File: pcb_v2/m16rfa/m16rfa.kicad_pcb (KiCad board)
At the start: 2 copper layers, 140.3 x 146.7 mm, 51 parts, among them J1 S16A, J10 bus_rf16_3, J2 S16A, J3 SWRDA, J5 S16A, J6 S16A, J7 S16A, J8 bus_rf16_1, J9 bus_rf16_2, U1 74LS125, U10 74LS244, U11 74LS244, U2 74LS193, U3 74LS138, U4 74LS08, U5 74LS04, U6 74LS08, U7 74LS244, U8 74LS244, U9 74LS244

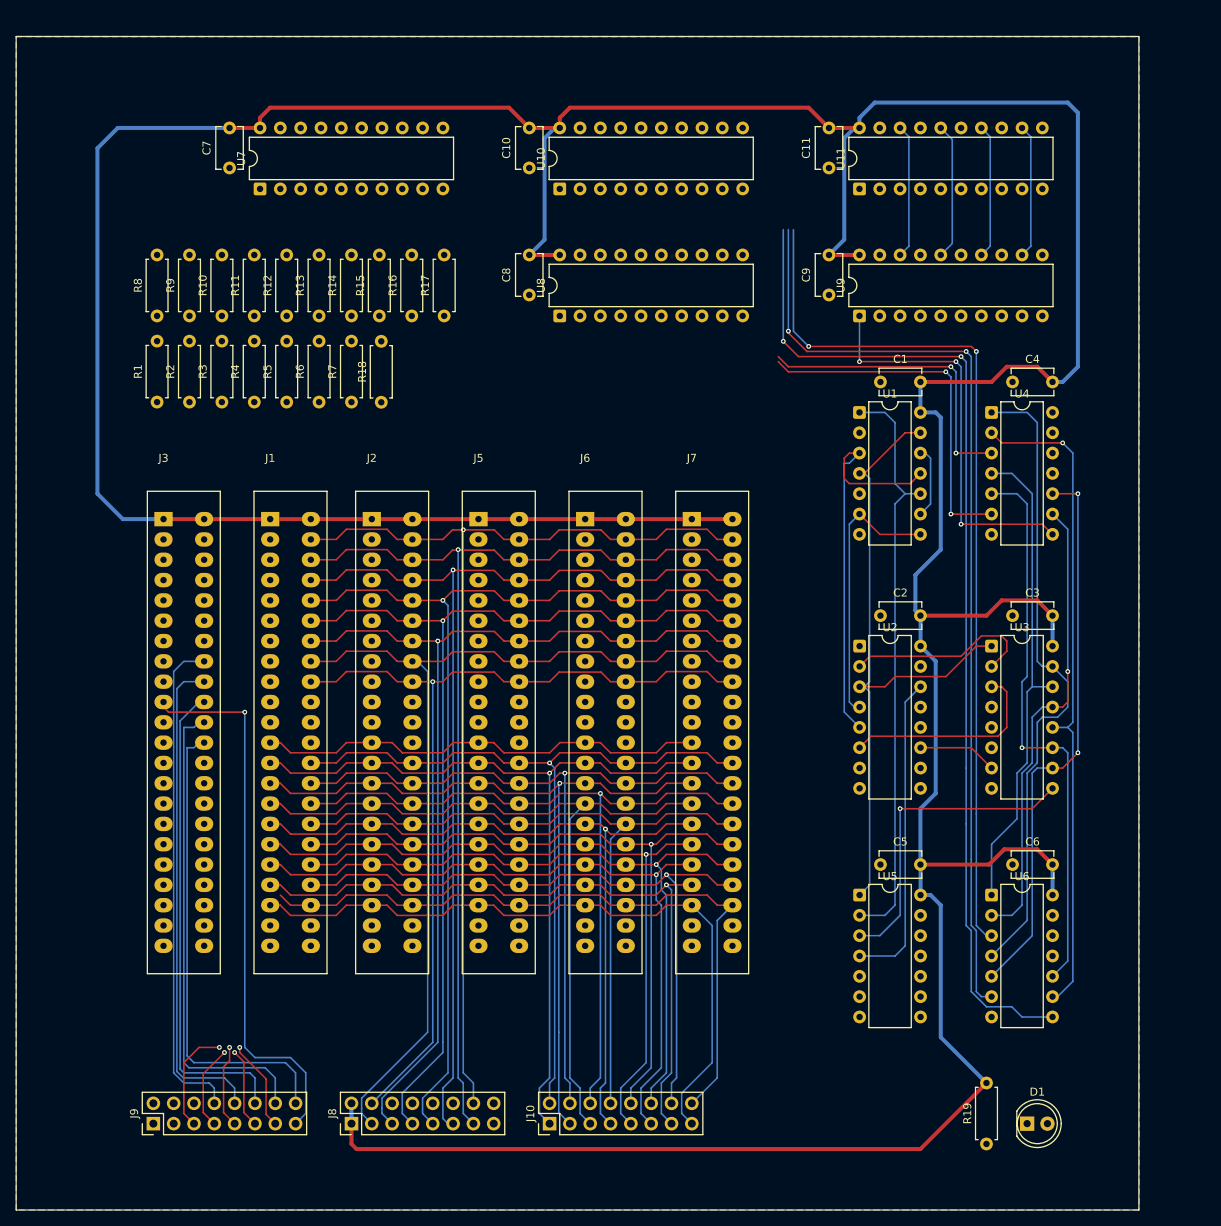
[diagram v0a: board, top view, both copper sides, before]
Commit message: recomeçando o roteamento
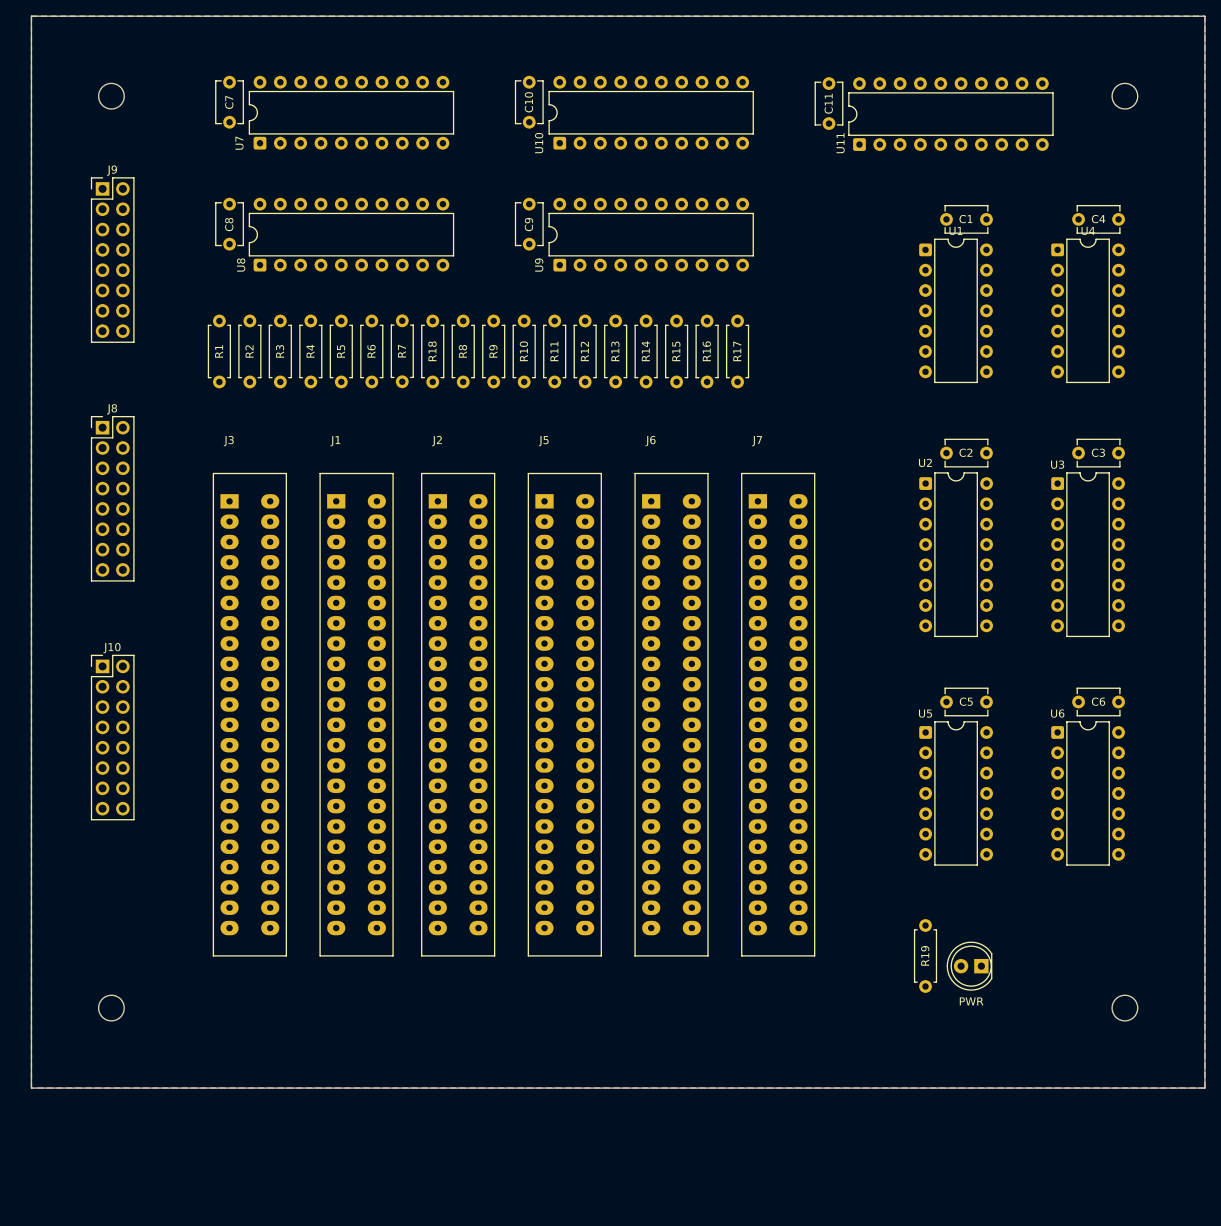
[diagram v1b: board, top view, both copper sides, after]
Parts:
- moved J9 117.0 mm to (36.8, 39.4), turned to 0 degrees
- moved J8 92.4 mm to (36.8, 69.2), turned to 0 degrees
- moved J10 79.9 mm to (36.8, 99.1), turned to 0 degrees
- moved R8 39.2 mm to (81.9, 63.5)
- moved R9 38.9 mm to (85.7, 63.5)
- moved R10 38.7 mm to (89.5, 63.5)
- moved R11 38.4 mm to (93.3, 63.5)
- moved R12 38.2 mm to (97.2, 63.5)
- moved R15 38.1 mm to (108.6, 63.5)
- moved C8 38.0 mm to (52.7, 46.3)
- moved C9 38.0 mm to (90.2, 46.3)
- moved U8 38.0 mm to (56.5, 48.9)
- moved U9 38.0 mm to (94.0, 48.9)
- moved R13 38.0 mm to (101.0, 63.5)
- moved R16 37.8 mm to (112.4, 63.5)
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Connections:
- J8 pad 11: data_{2} -> data_{5}
- J8 pad 13: data_{1} -> data_{6}
- J8 pad 14: data_{0} -> data_{7}
- J8 pad 3: data_{6} -> data_{1}
- J8 pad 4: data_{7} -> data_{0}
- J8 pad 5: data_{5} -> data_{2}
- J8 pad 7: data_{4} -> data_{3}
- J8 pad 9: data_{3} -> data_{4}
- U4 pad 12: unconnected-(U4-Pad12) -> +5V
- U4 pad 13: unconnected-(U4-Pad13) -> +5V
- U5 pad 11: unconnected-(U5-Pad11) -> +5V
- U5 pad 13: unconnected-(U5-Pad13) -> +5V
- U5 pad 5: unconnected-(U5-Pad5) -> +5V
- U5 pad 9: unconnected-(U5-Pad9) -> +5V
- U6 pad 12: unconnected-(U6-Pad12) -> +5V
- U6 pad 13: unconnected-(U6-Pad13) -> +5V
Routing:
- net +5V: track 582.5 -> 0.00 mm
- net data_{1}: track 130.0 -> 0.00 mm, vias 1 -> 0
- net data_{0}: track 129.7 -> 0.00 mm, vias 1 -> 0
- net data_{2}: track 128.7 -> 0.00 mm, vias 1 -> 0
- net lr_at_two: track 128.4 -> 0.00 mm, vias 2 -> 0
- net data_{3}: track 124.9 -> 0.00 mm, vias 1 -> 0
- net data_{4}: track 122.9 -> 0.00 mm, vias 1 -> 0
- net data_{5}: track 121.2 -> 0.00 mm, vias 1 -> 0
- net data_{6}: track 120.3 -> 0.00 mm
- net lr_at_one: track 118.8 -> 0.00 mm, vias 2 -> 0
- net data_{7}: track 113.3 -> 0.00 mm, vias 1 -> 0
- net lr_at_zero: track 110.8 -> 0.00 mm, vias 2 -> 0
- net addr_{1}: track 102.4 -> 0.00 mm, vias 1 -> 0
- net addr_{3}: track 100.7 -> 0.00 mm, vias 1 -> 0
- net addr_{0}: track 100.6 -> 0.00 mm, vias 1 -> 0
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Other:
- board size 140.3 x 146.7 mm -> 146.7 x 134 mm
